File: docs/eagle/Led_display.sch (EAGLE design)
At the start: 44 parts, among them Q1 16 Mhz, U1 328P, U2 LM317

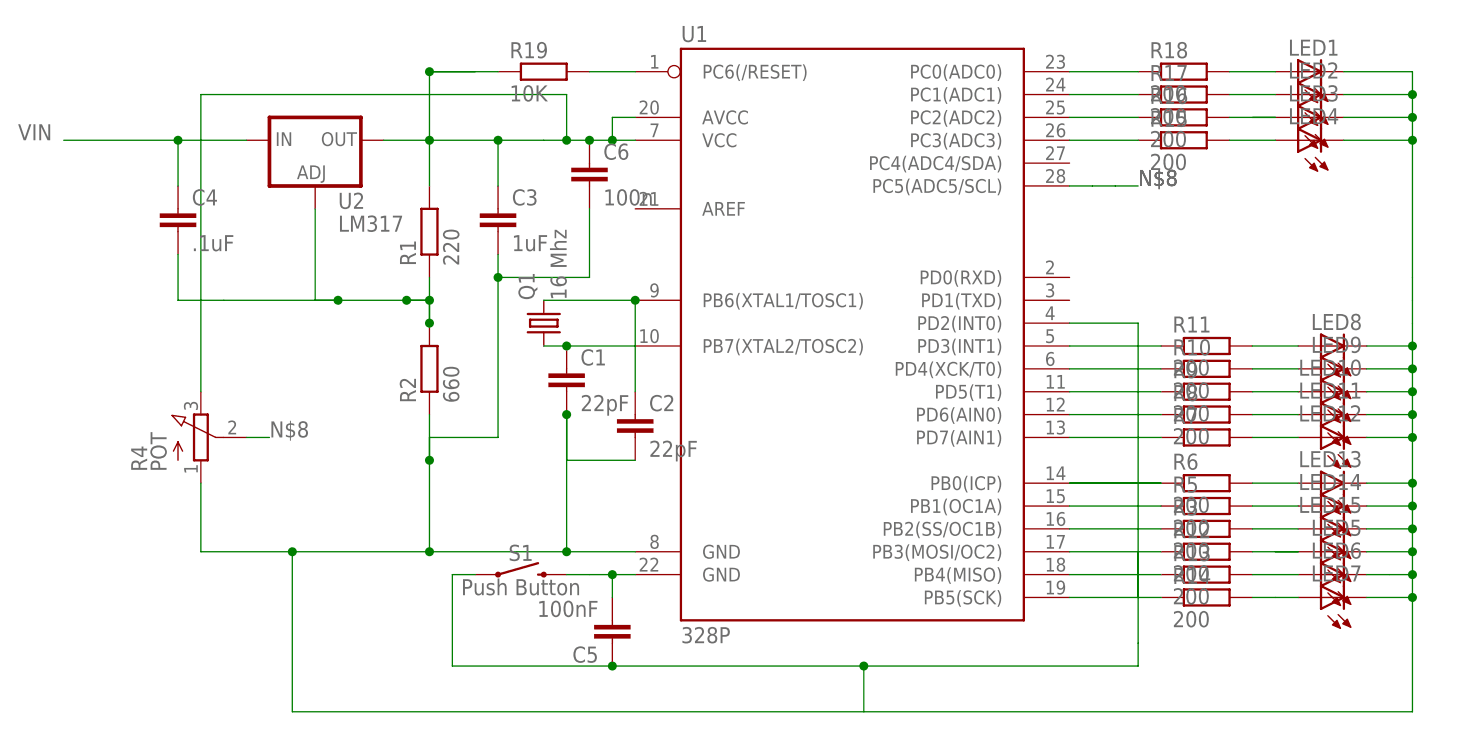
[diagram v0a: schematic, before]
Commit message: adjusting schematic
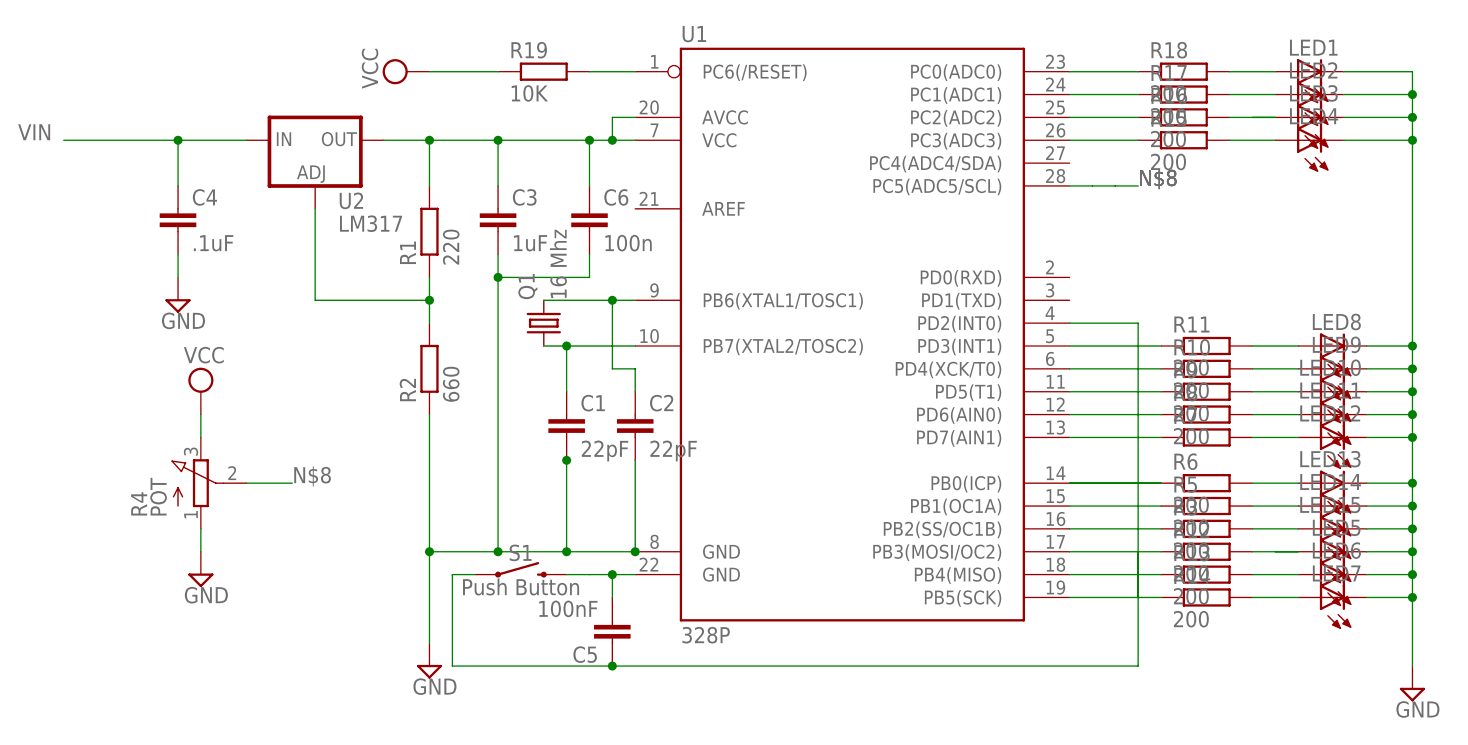
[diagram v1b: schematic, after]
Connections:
- removed net N$41 (its old number): C3.1, C6.1, R1.2, R19.1, R4.E, U1.AVCC, U1.VCC, U2.OUT
- removed net N$6: C4.2, R1.1, R2.2, U2.ADJ
- new net GND: C1.2, C2.2, C3.2, C4.2, C6.2, LED1.C, LED10.C, LED11.C, LED12.C, LED13.C, LED14.C, LED15.C, LED2.C, LED3.C, LED4.C, LED5.C, LED6.C, LED7.C, LED8.C, LED9.C, R2.1, R4.A, U1.GND@1
- new net N$4: R1.1, R2.2, U2.ADJ
- new net VCC: R19.1, R4.E
- net N$3: now also C3.1, C6.1, R1.2, U1.AVCC, U1.VCC, U2.OUT; no longer C1.2, C2.2, C3.2, C6.2, LED1.C, LED10.C, LED11.C, LED12.C, LED13.C, LED14.C, LED15.C, LED2.C, LED3.C, LED4.C, LED5.C, LED6.C, LED7.C, LED8.C, LED9.C, R2.1, R4.A, U1.GND@1
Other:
- moved on the sheet: C1, C6, R4
